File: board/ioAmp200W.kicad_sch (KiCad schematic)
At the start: 42 parts, among them J4 SM03B-SRSS-TB, SW1 SW_Push, SW2 SW_Push, U1 RP2350_60QFN, U2 TPS26750SRSMR, U3 TPD4S480RUKR, U4 ADAU1761BCPZ-RL, Y1 ABM8-272-T3

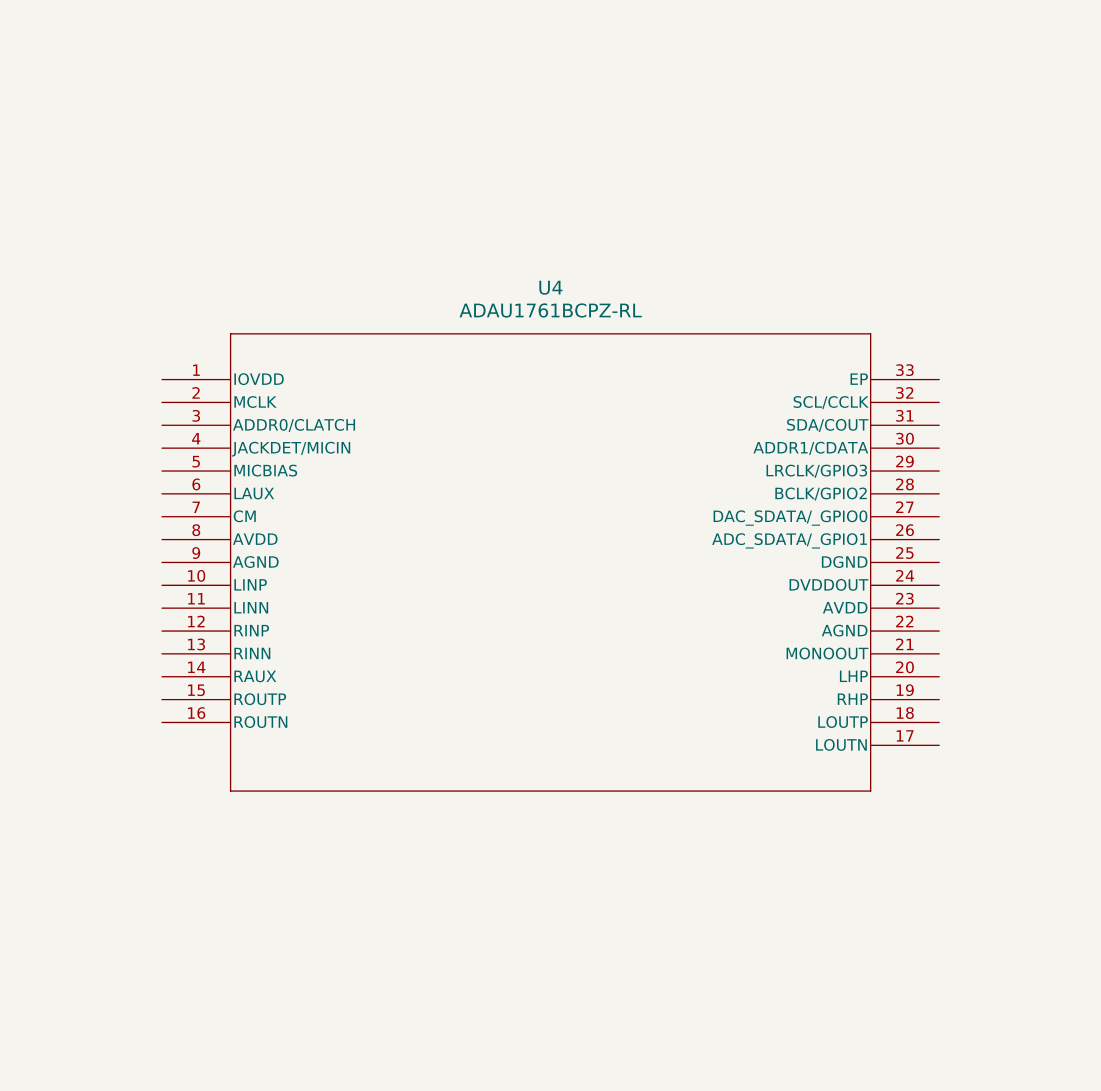
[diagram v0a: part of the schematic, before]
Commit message: switch_dsp
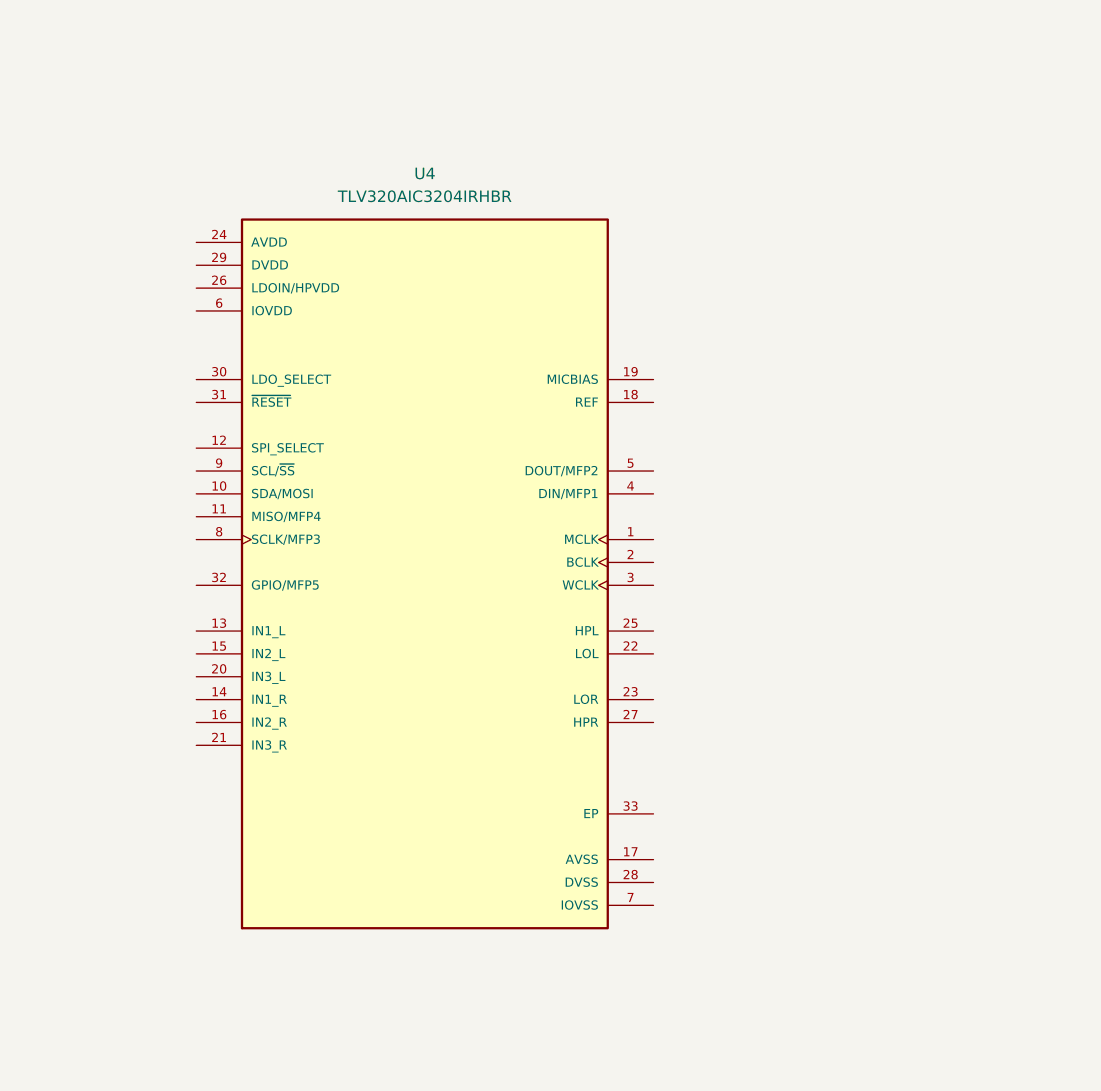
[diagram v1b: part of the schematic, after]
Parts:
- removed U4: ADAU1761BCPZ-RL, adau1761:CP-32-4_ADI, symbol adau1761:ADAU1761BCPZ-RL
- added U4: TLV320AIC3204IRHBR, TLV320AIC3204IRHBR:QFN50P500X500X100-33N, symbol TLV320AIC3204IRHBR:TLV320AIC3204IRHBR
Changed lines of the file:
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@@
-	)
-	(symbol
-		(lib_id "adau1761:ADAU1761BCPZ-RL")
-		(at 152.4 434.34 0)
-		(unit 1)
-		(exclude_from_sim no)
-		(in_bom yes)
-		(on_board yes)
-		(dnp no)
-		(fields_autoplaced yes)
-		(property "Reference" "U4"
-			(at 195.58 424.18 0)
-			(effects
-				(font
-					(size 1.524 1.524)
-				)
-			)
-		)
-		(property "Value" "ADAU1761BCPZ-RL"
-			(at 195.58 426.72 0)
-			(effects
-				(font
-					(size 1.524 1.524)
-				)
-			)
-		)
-		(property "Footprint" "adau1761:CP-32-4_ADI"
-			(at 152.4 434.34 0)
-			(effects
-				(font
-					(size 1.27 1.27)
-					(italic yes)
-				)
-				(hide yes)
-			)
-		)
-		(property "Datasheet" "https://www.analog.com/media/en/technical-documentation/data-sheets/ADAU1761.pdf"
-			(at 152.4 434.34 0)
-			(effects
-				(font
-					(size 1.27 1.27)
-					(italic yes)
-				)
-				(hide yes)
-			)
-		)
-		(property "Description" ""
-			(at 152.4 434.34 0)
-			(effects
-				(font
-					(size 1.27 1.27)
-				)
-				(hide yes)
-			)
-		)
-		(pin "17"
-		)
-		(pin "18"
-		)
-		(pin "19"
-		)
-		(pin "20"
-		)
-		(pin "21"
-		)
-		(pin "22"
-		)
-		(pin "23"
-		)
-		(pin "24"
-		)
-		(pin "25"
-		)
-		(pin "6"
-		)
-		(pin "5"
-		)
-		(pin "4"
-		)
-		(pin "3"
-		)
-		(pin "2"
-		)
-		(pin "1"
-		)
-		(pin "11"
-		)
-		(pin "10"
-		)
-		(pin "9"
-		)
-		(pin "8"
-		)
-		(pin "7"
-		)
-		(pin "12"
-		)
-		(pin "13"
-		)
-		(pin "14"
-		)
-		(pin "15"
-		)
-		(pin "16"
-		)
-		(pin "26"
-		)
-		(pin "27"
-		)
-		(pin "28"
-		)
-		(pin "29"
-		)
-		(pin "30"
-		)
-		(pin "31"
-		)
-		(pin "32"
-		)
-		(pin "33"
-		)
-		(instances
-			(project ""
-				(path "/4f3b51aa-8e6e-4521-ad6c-a7e6e194e2a4"
-					(reference "U4")
-					(unit 1)
-				)
-			)
-		)
 	)
 	(symbol
@@
 					(unit 1)
 				)
+			)
+		)
+	)
+	(symbol
+		(lib_id "TLV320AIC3204IRHBR:TLV320AIC3204IRHBR")
+		(at 181.61 454.66 0)
+		(unit 1)
+		(exclude_from_sim no)
+		(in_bom yes)
+		(on_board yes)
+		(dnp no)
+		(fields_autoplaced yes)
+		(property "Reference" "U4"
+			(at 181.61 411.48 0)
+			(effects
+				(font
+					(size 1.27 1.27)
+				)
+			)
+		)
+		(property "Value" "TLV320AIC3204IRHBR"
+			(at 181.61 414.02 0)
+			(effects
+				(font
+					(size 1.27 1.27)
+				)
+			)
+		)
+		(property "Footprint" "TLV320AIC3204IRHBR:QFN50P500X500X100-33N"
+			(at 181.61 454.66 0)
+			(effects
+				(font
+					(size 1.27 1.27)
+				)
+				(justify bottom)
+				(hide yes)
+			)
+		)
+		(property "Datasheet" ""
+			(at 181.61 454.66 0)
+			(effects
+				(font
+					(size 1.27 1.27)
+				)
+				(hide yes)
+			)
+		)
+		(property "Description" ""
+			(at 181.61 454.66 0)
+			(effects
+				(font
+					(size 1.27 1.27)
+				)
+				(hide yes)
+			)
+		)
+		(property "PARTREV" "E"
+			(at 181.61 454.66 0)
+			(effects
+				(font
+					(size 1.27 1.27)
+				)
+				(justify bottom)
+				(hide yes)
+			)
+		)
+		(property "STANDARD" "IPC-7351B"
+			(at 181.61 454.66 0)
+			(effects
+				(font
+					(size 1.27 1.27)
+				)
+				(justify bottom)
+				(hide yes)
+			)
+		)
+		(property "MAXIMUM_PACKAGE_HEIGHT" "1.0mm"
+			(at 181.61 454.66 0)
+			(effects
+				(font
+					(size 1.27 1.27)
+				)
+				(justify bottom)
+				(hide yes)
+			)
+		)
+		(property "MANUFACTURER" "Texas Instruments"
+			(at 181.61 454.66 0)
+			(effects
+				(font
+					(size 1.27 1.27)
+				)
+				(justify bottom)
+				(hide yes)
+			)
+		)
+		(pin "32"
+		)
+		(pin "13"
+		)
+		(pin "11"
+		)
+		(pin "8"
+		)
+		(pin "10"
+		)
+		(pin "30"
+		)
+		(pin "9"
+		)
+		(pin "29"
+		)
+		(pin "24"
+		)
+		(pin "26"
+		)
+		(pin "31"
+		)
+		(pin "15"
+		)
+		(pin "12"
+		)
+		(pin "5"
+		)
+		(pin "21"
+		)
+		(pin "20"
+		)
+		(pin "19"
+		)
+		(pin "6"
+		)
+		(pin "16"
+		)
+		(pin "18"
+		)
+		(pin "14"
+		)
+		(pin "33"
+		)
+		(pin "1"
+		)
+		(pin "27"
+		)
+		(pin "28"
+		)
+		(pin "25"
+		)
+		(pin "2"
+		)
+		(pin "17"
+		)
+		(pin "3"
+		)
+		(pin "23"
+		)
+		(pin "7"
+		)
+		(pin "4"
+		)
+		(pin "22"
+		)
+		(instances
+			(project ""
+				(path "/4f3b51aa-8e6e-4521-ad6c-a7e6e194e2a4"
+					(reference "U4")
+					(unit 1)
+				)
